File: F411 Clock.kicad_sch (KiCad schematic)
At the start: 26 parts, among them J1 USB_C_Receptacle_USB2.0_16P, Q1 DMG3415U, Q2 BC547, SW1 SW_Push, SW2 SW_Push, SW3 SW_Push, SW4 SW_Push, U1 STM32F411CCUx

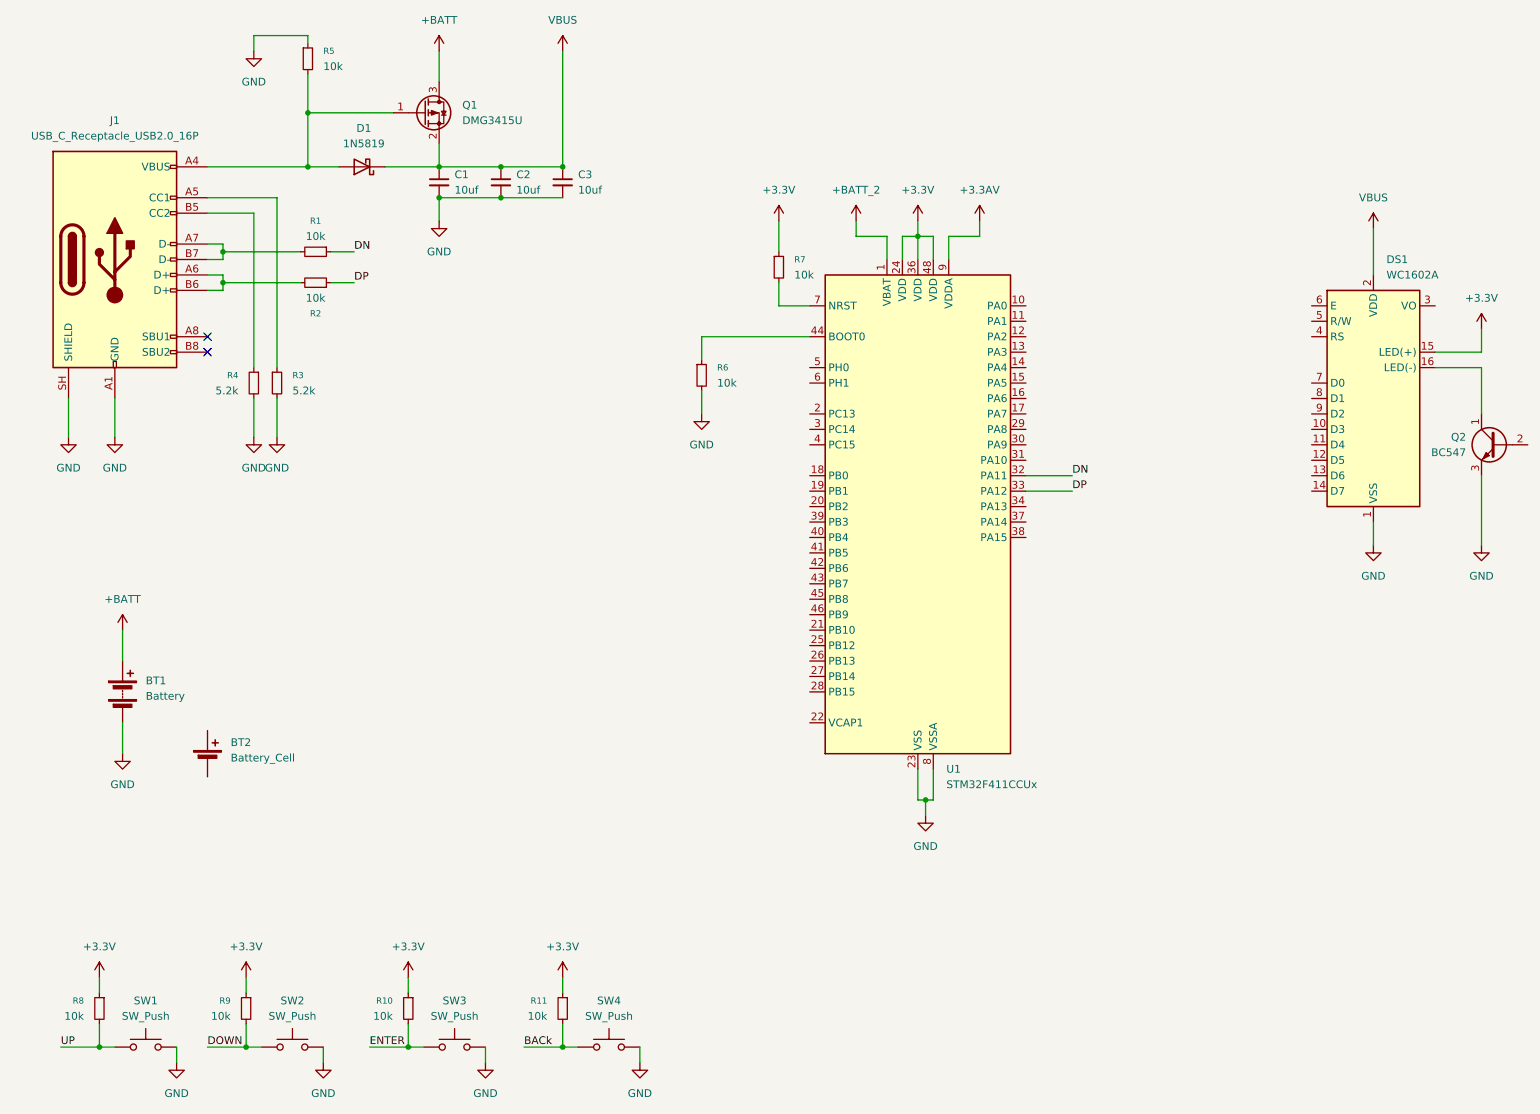
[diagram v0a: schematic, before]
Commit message: Discard unsaved pcb changes
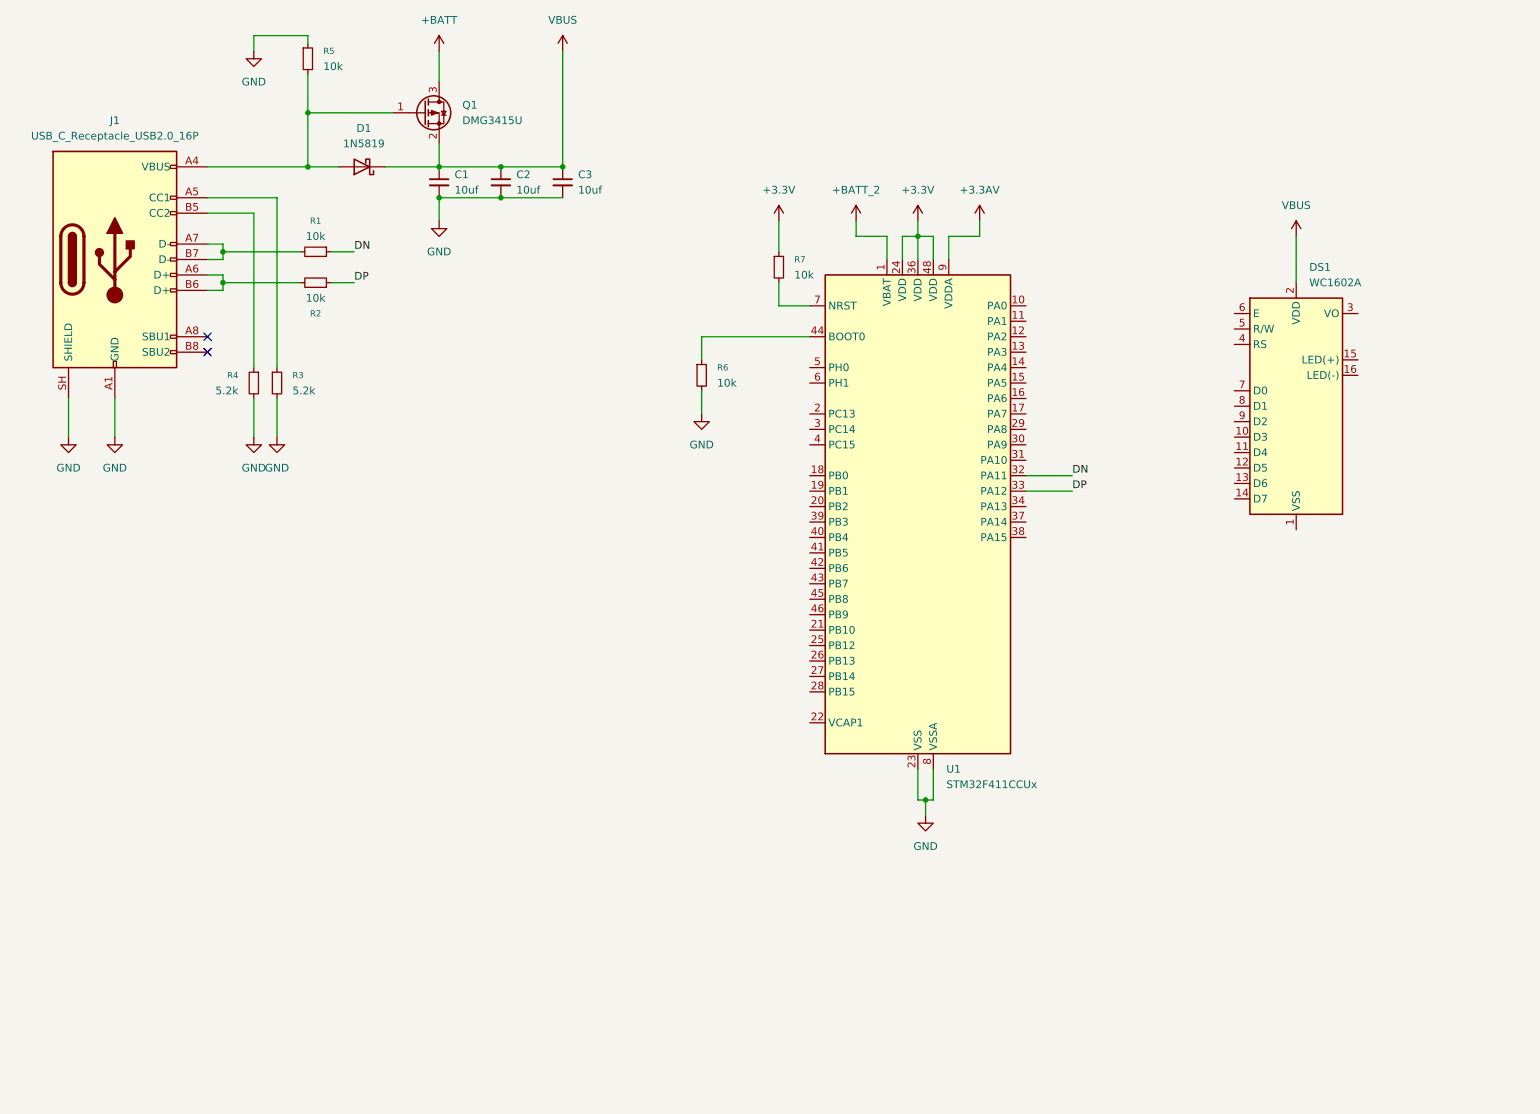
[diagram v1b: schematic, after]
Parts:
- removed BT1: Battery, Battery:BatteryHolder_Keystone_1042_1x18650, symbol Device:Battery
- removed BT2: Battery_Cell, Battery:BatteryHolder_Keystone_3034_1x20mm, symbol Device:Battery_Cell
- removed Q2: BC547, Package_TO_SOT_THT:TO-92L_Wide, symbol Transistor_BJT:BC547
- removed R10, R11, R8, R9: 10k, Resistor_SMD:R_0805_2012Metric, symbol Device:R_Small
- removed SW1, SW2, SW3, SW4: SW_Push, Button_Switch_SMD:SW_SPST_TL3342, symbol Switch:SW_Push
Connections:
- net +3.3V: no longer DS1.15 (LED(+))
- net GND: no longer DS1.1 (VSS)
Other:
- moved on the sheet: DS1

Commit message: SCH Save: 5 files changed .gitignore 3/0/0 F411 Clock.kicad_pro 0/0/1 F411 Clock.kicad_sch 3247/0/1089 ~F411 Clock.kicad_pcb.lck 0/1/0 ~F411 Clock.kicad_pro.lck 1/0/0
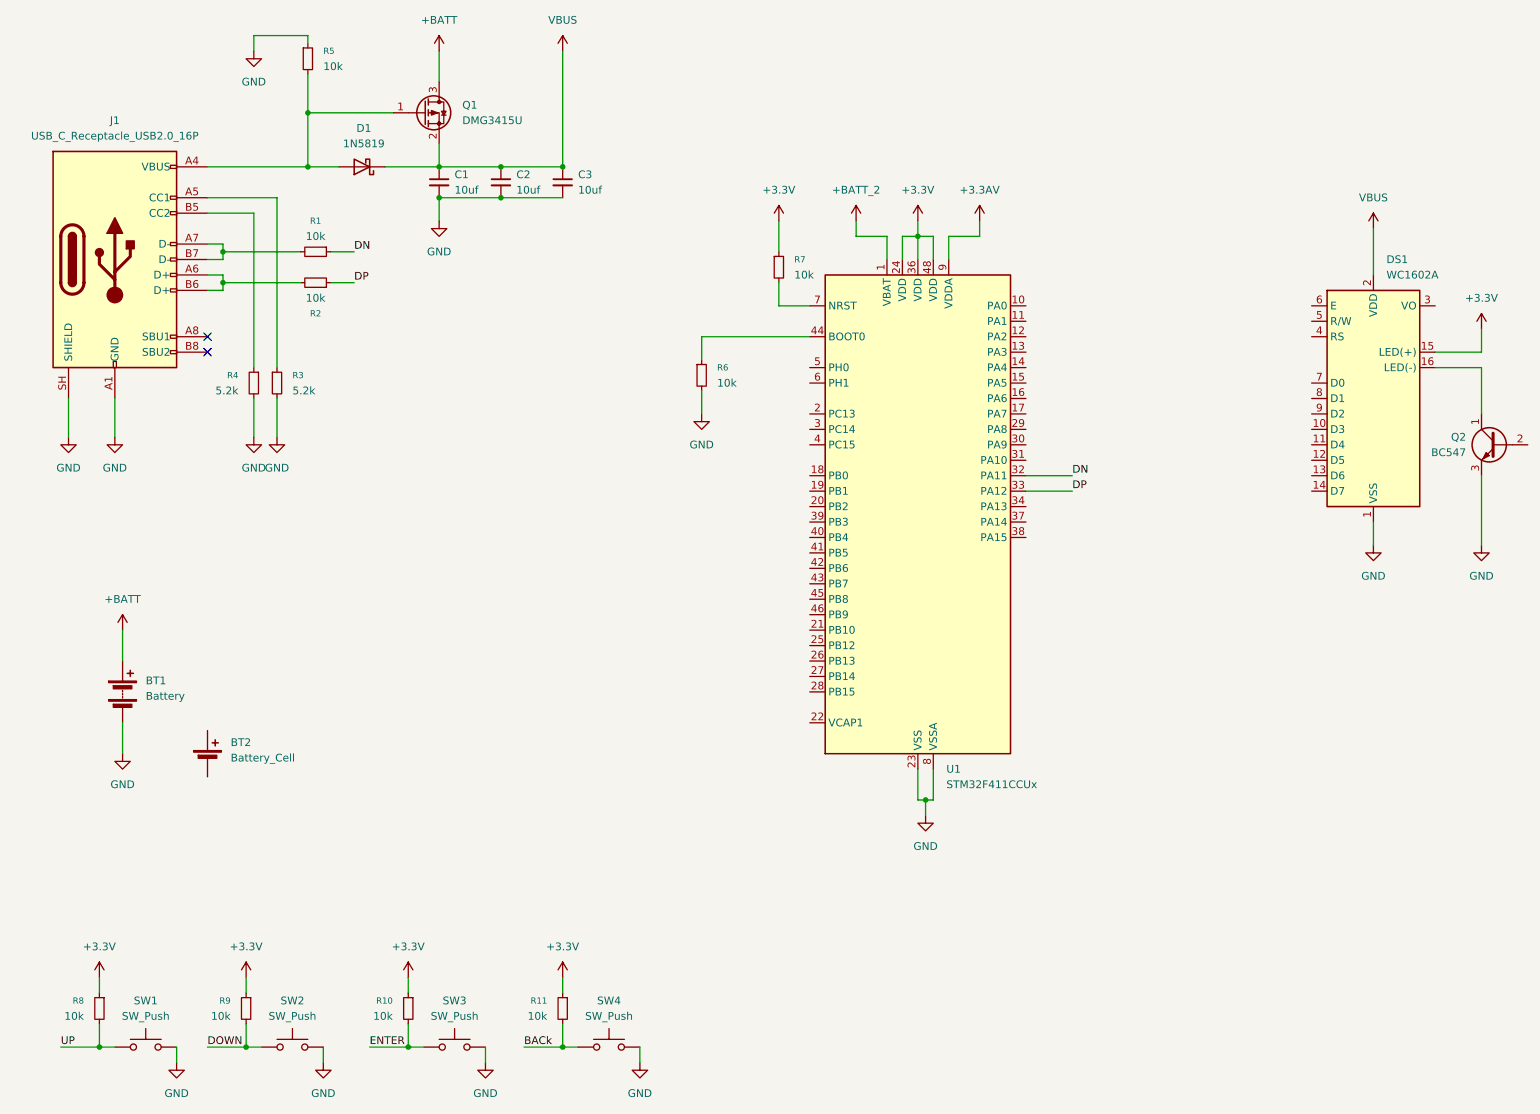
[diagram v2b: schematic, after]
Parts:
- added BT1: Battery, Battery:BatteryHolder_Keystone_1042_1x18650, symbol Device:Battery
- added BT2: Battery_Cell, Battery:BatteryHolder_Keystone_3034_1x20mm, symbol Device:Battery_Cell
- added Q2: BC547, Package_TO_SOT_THT:TO-92L_Wide, symbol Transistor_BJT:BC547
- added R10, R11, R8, R9: 10k, Resistor_SMD:R_0805_2012Metric, symbol Device:R_Small
- added SW1, SW2, SW3, SW4: SW_Push, Button_Switch_SMD:SW_SPST_TL3342, symbol Switch:SW_Push
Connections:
- net +3.3V: now also DS1.15 (LED(+)), R10.1, R11.1, R8.1, R9.1
- net +BATT: now also BT1.1 (+)
- net GND: now also DS1.1 (VSS), BT1.2 (-), Q2.3 (E), SW1.2, SW2.2, SW3.2, SW4.2
- net at DS1.16 (LED(-)): now also Q2.1 (C)
- new net BACk: R11.2, SW4.1
- new net DOWN: R9.2, SW2.1
- new net ENTER: R10.2, SW3.1
- new net UP: R8.2, SW1.1
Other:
- moved on the sheet: DS1
